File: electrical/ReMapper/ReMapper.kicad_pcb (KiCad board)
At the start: 4 copper layers, 32 x 55 mm, 42 parts, among them J1 ESP_UART0, J2 I2C Display, J3 USB_IN, J4 USB_OUT, J5 Button GND Pad, J9 Button Socket, U1 SPX1117M3-L-3-3/TR, U2 W25Q128JVE, U3 ESP32-S3-WROOM-1-N8R8, U4 RP2040, U5 W25Q128JVE, Y1 12MHZ

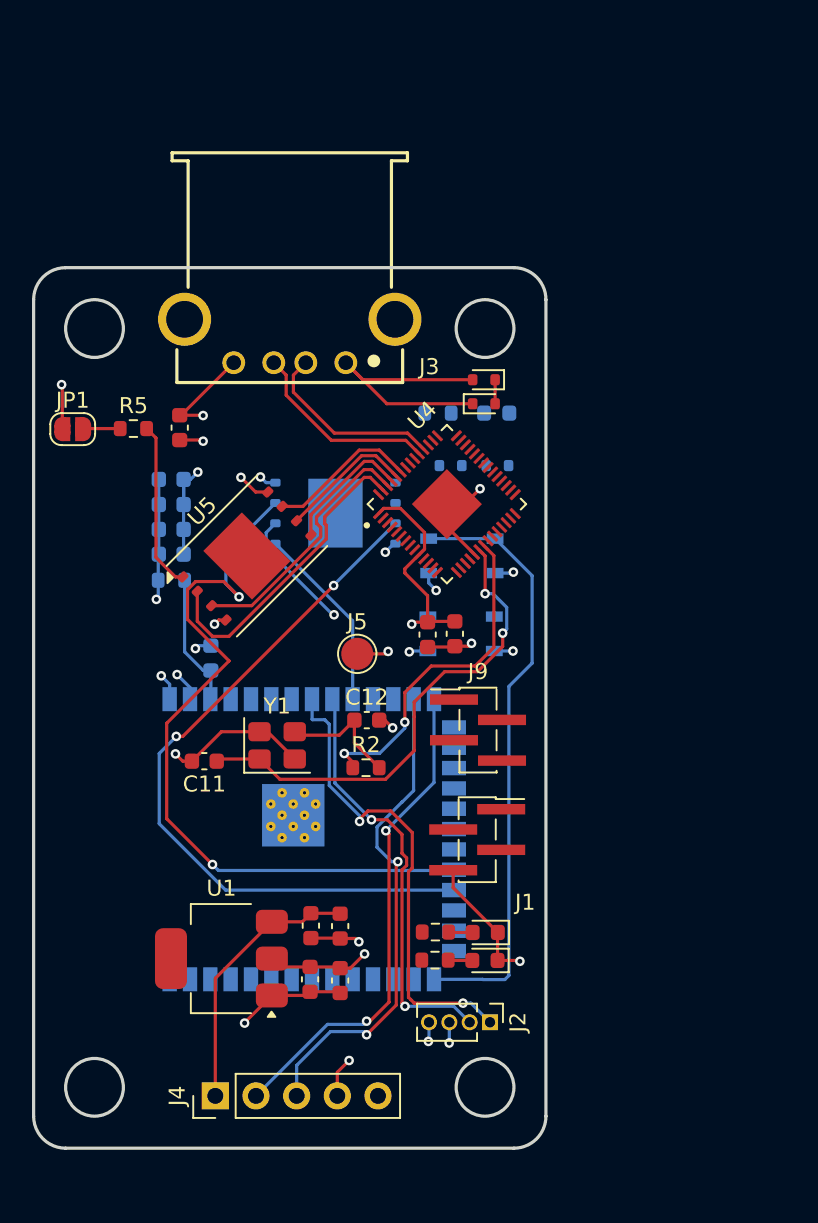
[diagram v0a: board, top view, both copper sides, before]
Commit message: way happier with this layout
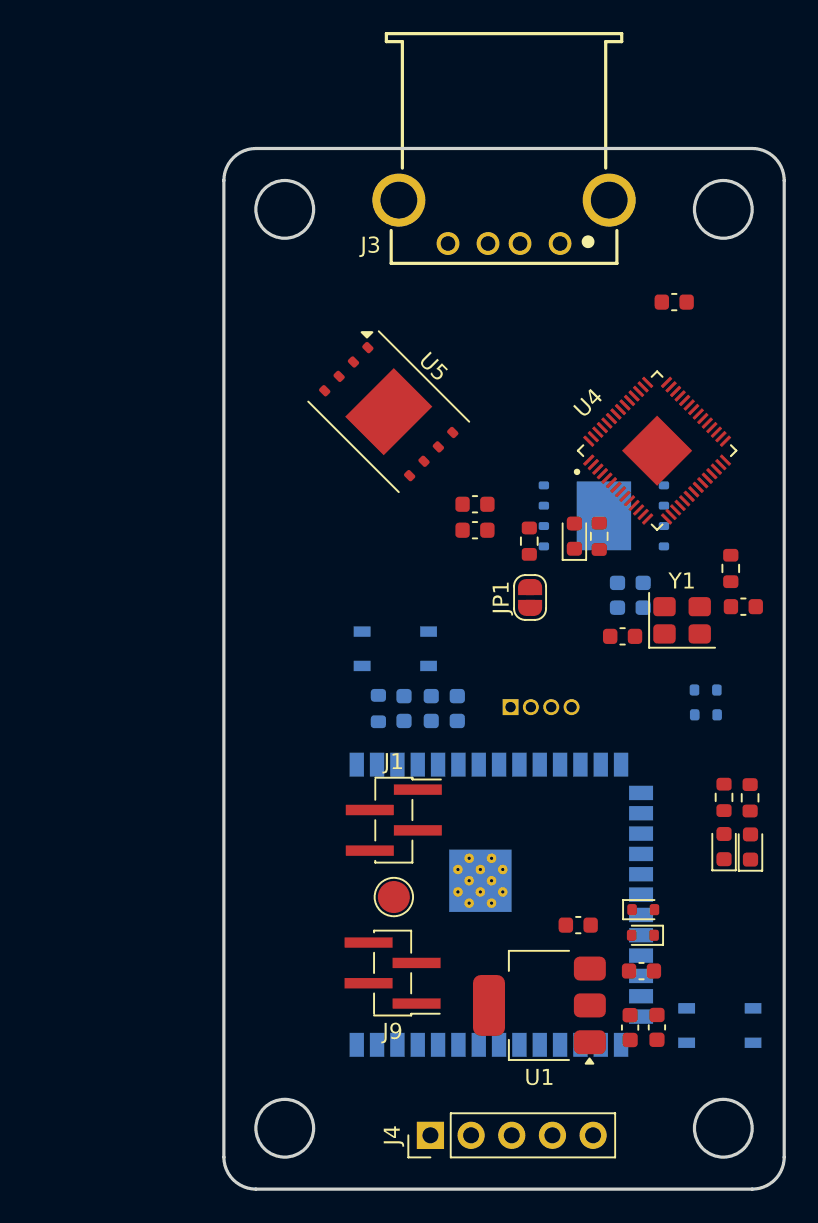
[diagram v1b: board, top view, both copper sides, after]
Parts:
- J2: moved to B.Cu
- LED1, R3: moved to F.Cu
- moved D2 36.1 mm to (204.0, 93.1)
- moved S2 33.5 mm to (208.9, 98.7), turned to 0 degrees
- moved D1 33.1 mm to (204.1, 91.5)
- moved C10 31.9 mm to (206.0, 53.5), turned to 0 degrees
- moved LED1 30.6 mm to (209.1, 87.5), turned to 90 degrees
- moved JP1 30.4 mm to (197.0, 72.0), turned to 90 degrees
- moved C5 30.0 mm to (204.1, 71.8), turned to -90 degrees
- moved R3 29.9 mm to (209.1, 84.5), turned to -90 degrees
- moved C6 28.8 mm to (202.5, 71.8), turned to -90 degrees
- moved R6 28.4 mm to (201.3, 68.1), turned to -90 degrees
- moved C11 27.3 mm to (202.8, 74.4)
- moved LED3 27.1 mm to (199.8, 68.1), turned to 90 degrees
- moved Y1 26.5 mm to (206.5, 73.4)
- moved R2 26.0 mm to (209.5, 70.2), turned to -90 degrees
- moved R5 25.7 mm to (197.0, 68.5), turned to 90 degrees
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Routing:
- net GND: track 70.4 -> 0.00 mm, vias 21 -> 0
- net /QSPI_IO2_esp: track 47.6 -> 0.00 mm, vias 2 -> 0
- net /QSPI_IO3_esp: track 45.2 -> 0.00 mm, vias 2 -> 0
- net /ESP_IO0: track 37.8 -> 0.00 mm
- net /3.3V: track 34.6 -> 0.00 mm, vias 8 -> 0
- net /USB_VIN: track 34.2 -> 0.00 mm
- net /USB_OUT_D-: track 31.0 -> 0.00 mm, vias 2 -> 0
- net /XIN_rp: track 30.8 -> 0.00 mm, vias 2 -> 0
- net /USB_OUT_D+: track 30.7 -> 0.00 mm, vias 2 -> 0
- net /I2C_DATA_DISPLAY: track 29.6 -> 0.00 mm, vias 2 -> 0
- net /I2C_CLK_DISPLAY: track 26.3 -> 0.00 mm, vias 2 -> 0
- net /XOUT_rp: track 21.2 -> 0.00 mm, vias 2 -> 0
- net /QSPI_IO1_rp: track 19.3 -> 0.00 mm
- net /QSPI_IO2_rp: track 16.0 -> 0.00 mm
- net /USB_IN_D+: track 12.2 -> 0.00 mm
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- removed copper zone on In2.Cu, net /3.3V
- removed copper zone on In1.Cu, net GND
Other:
- board size 32 x 55 mm -> 35 x 65 mm
